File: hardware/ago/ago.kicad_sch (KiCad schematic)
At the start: 17 parts

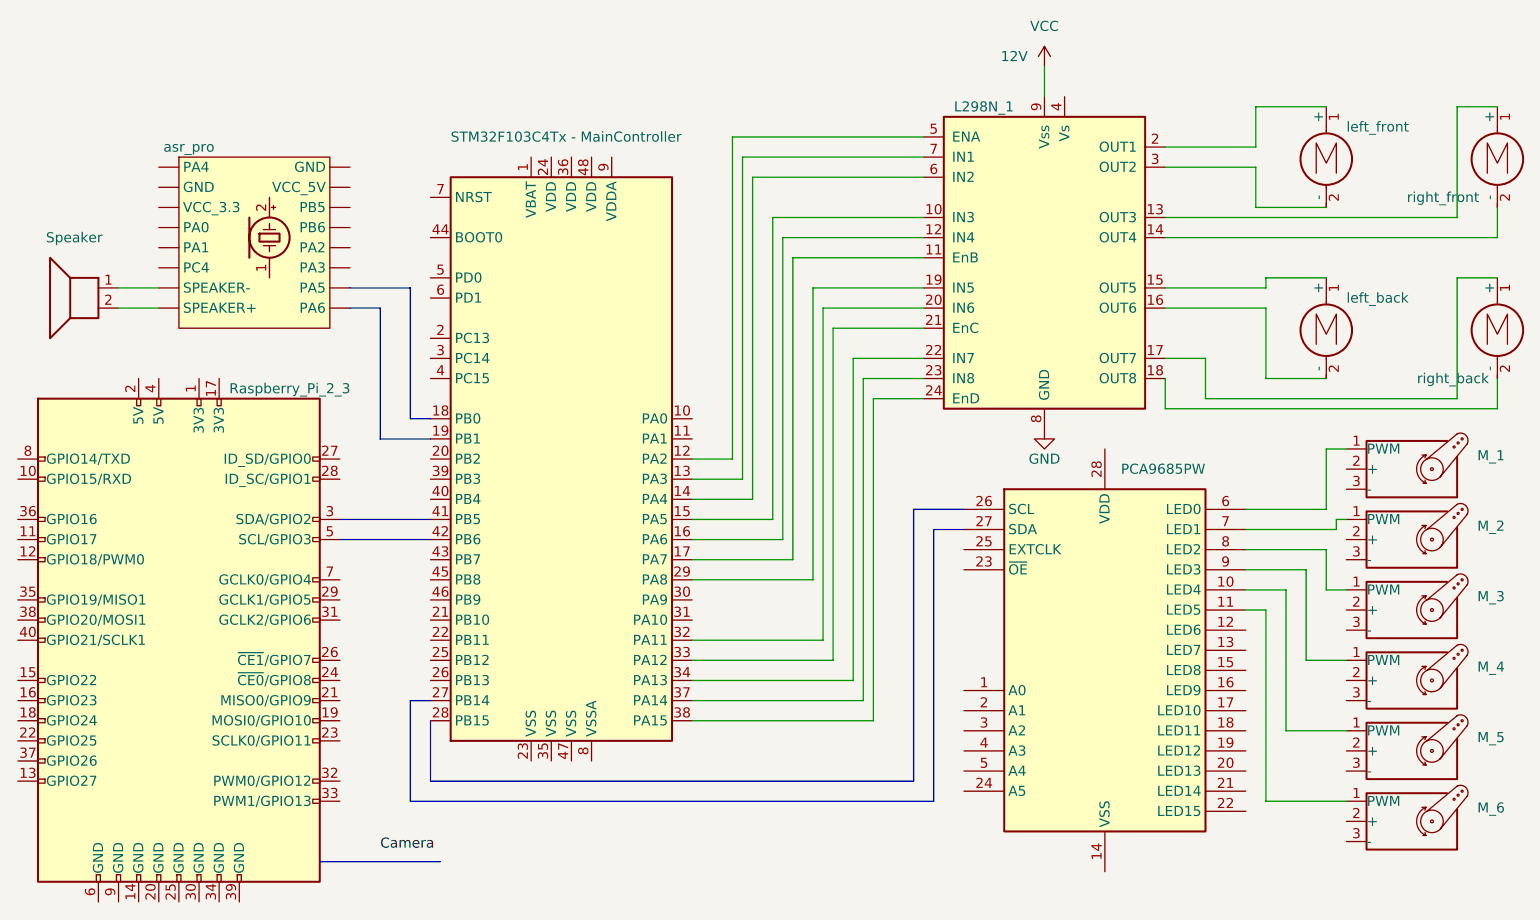
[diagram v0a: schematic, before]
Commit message: fix hardware design.
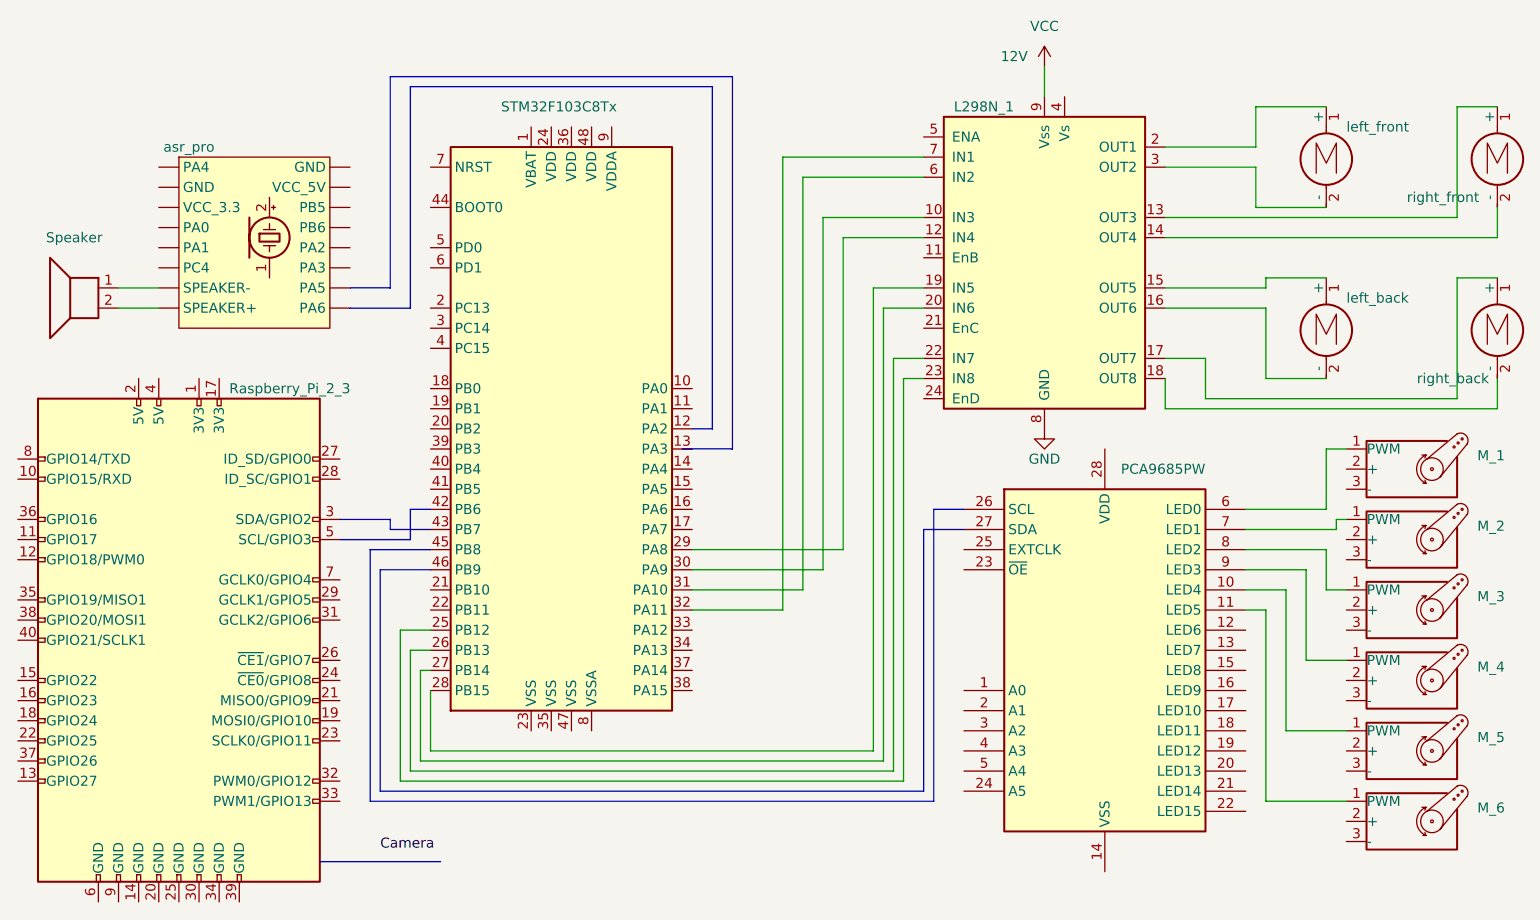
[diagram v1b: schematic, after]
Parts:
- removed U?: STM32F103C4Tx - MainController, Package_QFP:LQFP-48_7x7mm_P0.5mm, symbol MCU_ST_STM32F1:STM32F103C4Tx
- added U?: STM32F103C8Tx, Package_QFP:LQFP-48_7x7mm_P0.5mm, symbol MCU_ST_STM32F1:STM32F103C8Tx
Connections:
- net at U?.10 (IN3): now also U?.30 (PA9)
- net at U?.12 (IN4): now also U?.29 (PA8)
- net at U?.19 (IN5): now also U?.28 (PB15)
- net at U?.20 (IN6): now also U?.27 (PB14)
- net at U?.22 (IN7): now also U?.26 (PB13)
- net at U?.23 (IN8): now also U?.25 (PB12)
- net at U?.6 (IN2): now also U?.31 (PA10)
- net at U?.7 (IN1): now also U?.32 (PA11)
